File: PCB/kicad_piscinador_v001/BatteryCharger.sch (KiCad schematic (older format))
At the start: 0 parts

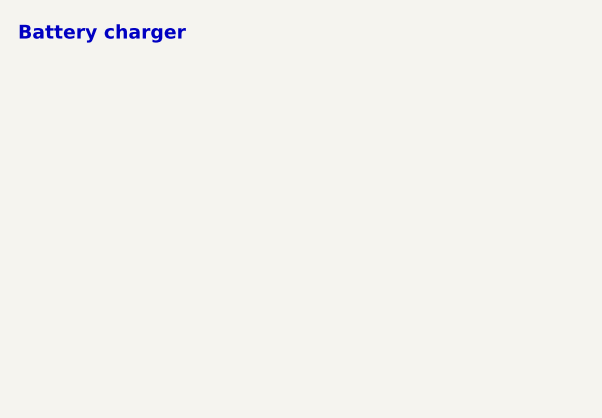
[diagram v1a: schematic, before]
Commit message: project backup
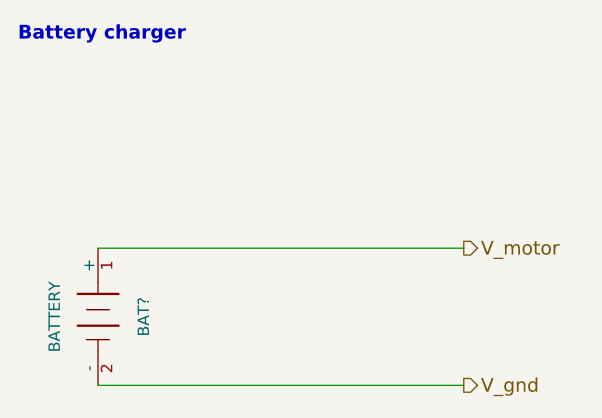
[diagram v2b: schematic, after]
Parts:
- added BAT?: BATTERY, symbol BATTERY
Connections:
- new net V_gnd: BAT?.2 (-)
- new net V_motor: BAT?.1 (+)
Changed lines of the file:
@@
 LIBS:Zilog
 LIBS:Common-Parts-Library
+LIBS:freetronics_schematic
 LIBS:kicad_test_picinador-cache
 EELAYER 25 0
@@
 Text Notes 3050 1800 0    60   ~ 12
 Battery charger
+$Comp
+L BATTERY BAT?
+U 1 1 57FFC7C9
+P 3400 3000
+F 0 "BAT?" H 3400 3200 50  0000 C CNN
+F 1 "BATTERY" H 3400 2810 50  0000 C CNN
+F 2 "" H 3400 3000 60  0000 C CNN
+F 3 "" H 3400 3000 60  0000 C CNN
+	1    3400 3000
+	0    1    1    0
+$EndComp
+Text HLabel 5000 2700 2    60   Output ~ 0
+V_motor
+Text HLabel 5000 3300 2    60   Output ~ 0
+V_gnd
+Wire Wire Line
+	5000 3300 3400 3300
+Wire Wire Line
+	3400 2700 5000 2700
 $EndSCHEMATC
